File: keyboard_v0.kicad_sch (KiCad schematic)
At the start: 21 parts, among them J1 AVR-ISP-6, J3 UJ20-C-H-G-SMT-1-P16-TR, SW1 SW_RESET, U1 ATmega32U4-A, U2 USBLC6-2P6, Y1 Crystal_GND24_Small

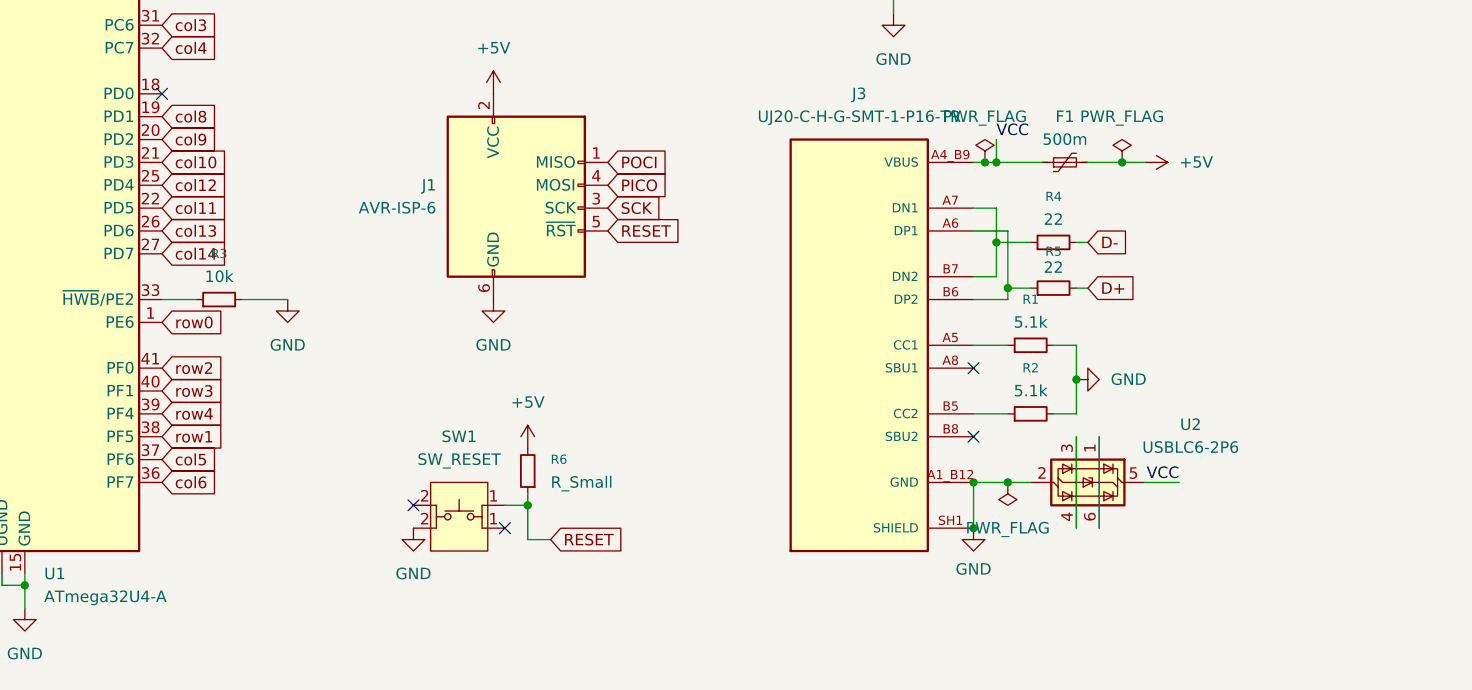
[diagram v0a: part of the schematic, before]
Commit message: Complete routing
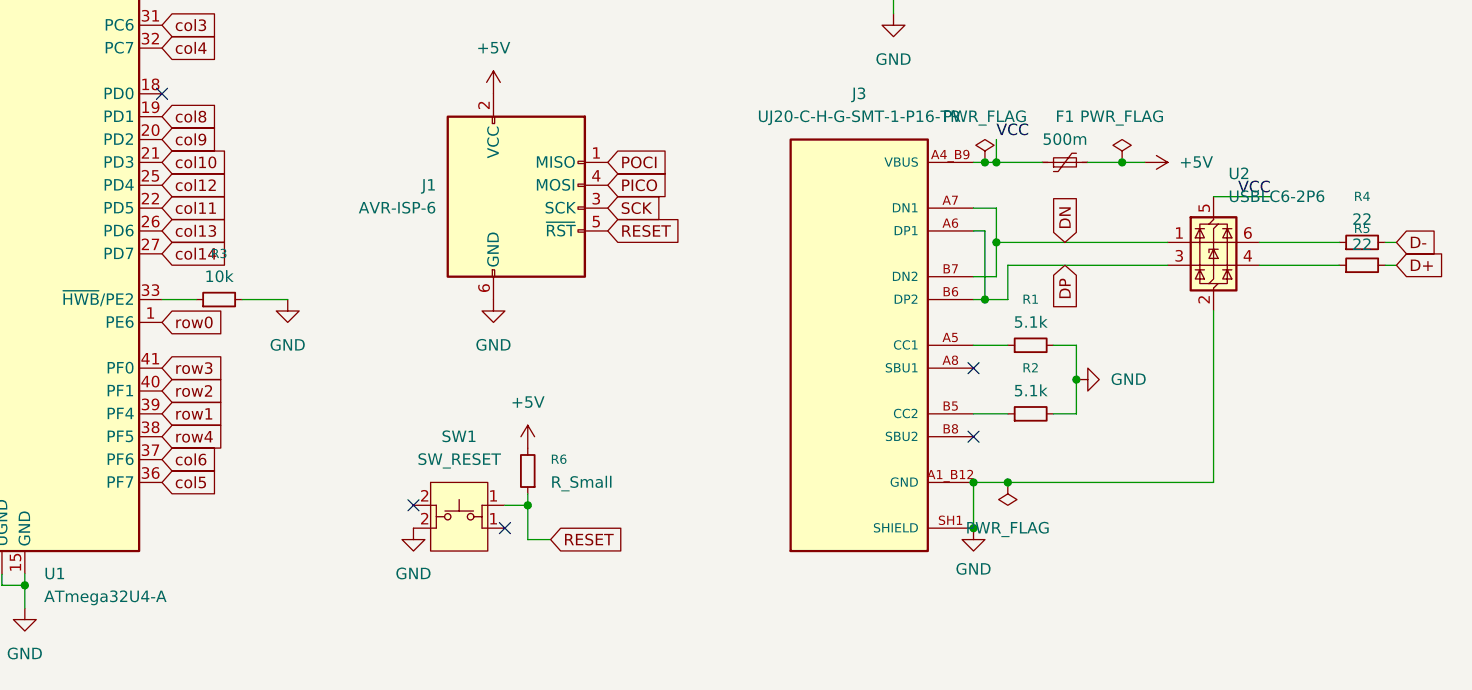
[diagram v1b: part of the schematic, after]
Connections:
- net col5: now also U1.36 (PF7); no longer U1.37 (PF6)
- net col6: now also U1.37 (PF6); no longer U1.36 (PF7)
- net row1: now also U1.39 (PF4); no longer U1.38 (PF5)
- net row2: now also U1.40 (PF1); no longer U1.41 (PF0)
- net row3: now also U1.41 (PF0); no longer U1.40 (PF1)
- net row4: now also U1.38 (PF5); no longer U1.39 (PF4)
- net DP: now reaches J3.A6 (DP1), J3.B6 (DP2)
- net DP: now also U2.3 (I/O2); no longer R5.1
- net DN: now reaches J3.A7 (DN1), J3.B7 (DN2)
- net DN: now also U2.1 (I/O1); no longer R4.1
- net at U2.6 (I/O1): now also R4.1; no longer U2.1 (I/O1)
- net at U2.4 (I/O2): now also R5.1; no longer U2.3 (I/O2)
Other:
- moved on the sheet: R4, R5, U2
